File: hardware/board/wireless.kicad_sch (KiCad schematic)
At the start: 1 part, among them J1 Bus_M.2_Socket_E

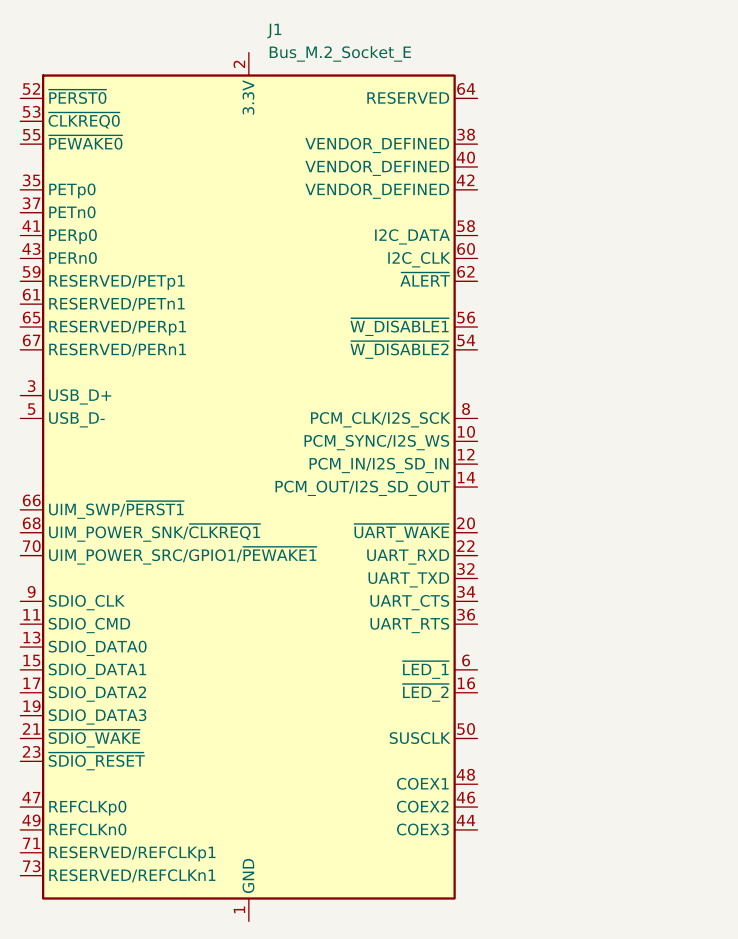
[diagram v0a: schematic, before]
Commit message: added stuff
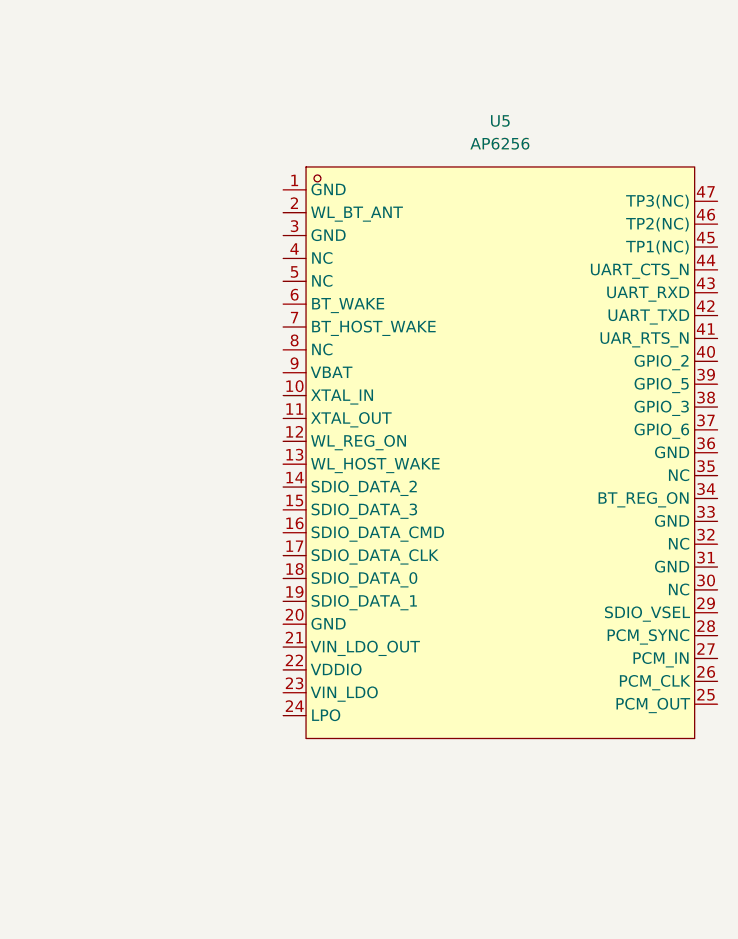
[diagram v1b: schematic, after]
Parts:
- removed J1: Bus_M.2_Socket_E, symbol Connector:Bus_M.2_Socket_E
- added U5: AP6256, lcsc:QFN-44_L12.0-W12.0-P0.90-TL_AP6256, symbol lcsc:AP6256
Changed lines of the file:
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@@
 	(paper "A4")
 	(symbol
-		(lib_id "Connector:Bus_M.2_Socket_E")
-		(at 219.71 90.17 0)
+		(lib_id "lcsc:AP6256")
+		(at 247.65 86.36 0)
 		(unit 1)
 		(exclude_from_sim no)
@@
 		(dnp no)
 		(fields_autoplaced yes)
-		(property "Reference" "J1"
-			(at 221.8533 39.37 0)
+		(property "Reference" "U5"
+			(at 247.65 49.53 0)
 			(effects
 				(font
 					(size 1.27 1.27)
 				)
-				(justify left)
 			)
 		)
-		(property "Value" "Bus_M.2_Socket_E"
-			(at 221.8533 41.91 0)
+		(property "Value" "AP6256"
+			(at 247.65 52.07 0)
 			(effects
 				(font
 					(size 1.27 1.27)
 				)
-				(justify left)
 			)
 		)
-		(property "Footprint" ""
-			(at 219.71 63.5 0)
+		(property "Footprint" "lcsc:QFN-44_L12.0-W12.0-P0.90-TL_AP6256"
+			(at 247.65 123.19 0)
 			(effects
 				(font
@@
 			)
 		)
-		(property "Datasheet" "https://web.archive.org/web/20200613074028/http://read.pudn.com/downloads794/doc/project/3133918/PCIe_M.2_Electromechanical_Spec_Rev1.0_Final_11012013_RS_Clean.pdf#page=150"
-			(at 219.71 77.47 0)
+		(property "Datasheet" ""
+			(at 247.65 86.36 0)
 			(effects
 				(font
@@
 			)
 		)
-		(property "Description" "M.2 Socket 1-SD Mechanical Key E"
-			(at 219.71 90.17 0)
+		(property "Description" ""
+			(at 247.65 86.36 0)
 			(effects
 				(font
@@
 			)
 		)
-		(pin "51"
+		(property "LCSC Part" "C5248079"
+			(at 247.65 125.73 0)
+			(effects
+				(font
+					(size 1.27 1.27)
+				)
+				(hide yes)
+			)
 		)
-		(pin "62"
+		(pin "28"
+		)
+		(pin "2"
+		)
+		(pin "3"
+		)
+		(pin "46"
+		)
+		(pin "38"
+		)
+		(pin "27"
+		)
+		(pin "43"
+		)
+		(pin "32"
+		)
+		(pin "10"
+		)
+		(pin "47"
+		)
+		(pin "4"
+		)
+		(pin "13"
+		)
+		(pin "37"
+		)
+		(pin "42"
+		)
+		(pin "44"
+		)
+		(pin "16"
+		)
+		(pin "9"
+		)
+		(pin "14"
+		)
+		(pin "22"
 		)
 		(pin "39"
 		)
-		(pin "69"
+		(pin "35"
 		)
-		(pin "41"
+		(pin "30"
 		)
-		(pin "66"
+		(pin "6"
 		)
-		(pin "67"
+		(pin "33"
+		)
+		(pin "1"
+		)
+		(pin "5"
+		)
+		(pin "26"
+		)
+		(pin "7"
+		)
+		(pin "12"
+		)
+		(pin "11"
 		)
 		(pin "17"
 		)
-		(pin "75"
+		(pin "18"
 		)
-		(pin "61"
+		(pin "40"
 		)
-		(pin "73"
+		(pin "15"
 		)
-		(pin "58"
+		(pin "20"
 		)
-		(pin "6"
+		(pin "19"
 		)
-		(pin "3"
+		(pin "31"
 		)
-		(pin "37"
+		(pin "34"
 		)
-		(pin "59"
+		(pin "24"
 		)
-		(pin "55"
-		)
-		(pin "13"
-		)
-		(pin "49"
+		(pin "8"
 		)
 		(pin "21"
@@
 		(pin "23"
 		)
-		(pin "35"
-		)
-		(pin "43"
-		)
-		(pin "68"
-		)
-		(pin "5"
-		)
-		(pin "15"
-		)
-		(pin "19"
-		)
-		(pin "47"
-		)
-		(pin "4"
-		)
-		(pin "74"
-		)
-		(pin "1"
-		)
-		(pin "52"
-		)
-		(pin "2"
-		)
-		(pin "18"
-		)
-		(pin "33"
-		)
-		(pin "70"
-		)
 		(pin "45"
 		)
-		(pin "63"
-		)
-		(pin "11"
-		)
-		(pin "65"
-		)
-		(pin "9"
-		)
-		(pin "7"
-		)
-		(pin "64"
-		)
-		(pin "38"
-		)
-		(pin "40"
-		)
-		(pin "57"
-		)
-		(pin "42"
-		)
-		(pin "53"
-		)
-		(pin "72"
-		)
-		(pin "71"
-		)
-		(pin "60"
-		)
-		(pin "56"
-		)
-		(pin "8"
-		)
-		(pin "10"
-		)
-		(pin "54"
-		)
-		(pin "12"
-		)
-		(pin "14"
-		)
-		(pin "22"
-		)
-		(pin "32"
-		)
-		(pin "34"
-		)
-		(pin "20"
+		(pin "41"
 		)
 		(pin "36"
 		)
-		(pin "16"
+		(pin "29"
 		)
-		(pin "50"
-		)
-		(pin "44"
-		)
-		(pin "48"
-		)
-		(pin "46"
+		(pin "25"
 		)
 		(instances
-			(project "frost"
+			(project ""
 				(path "/3bc38516-4fe0-4022-adb8-9fd55b66cd2d/8c9baa61-05fe-4ea8-9287-072748c6c20c"
-					(reference "J1")
+					(reference "U5")
 					(unit 1)
 				)
